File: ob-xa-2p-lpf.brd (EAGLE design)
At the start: 50.8 x 85.5 mm, 53 parts, among them IC1 AS3320, IC3 TL082P

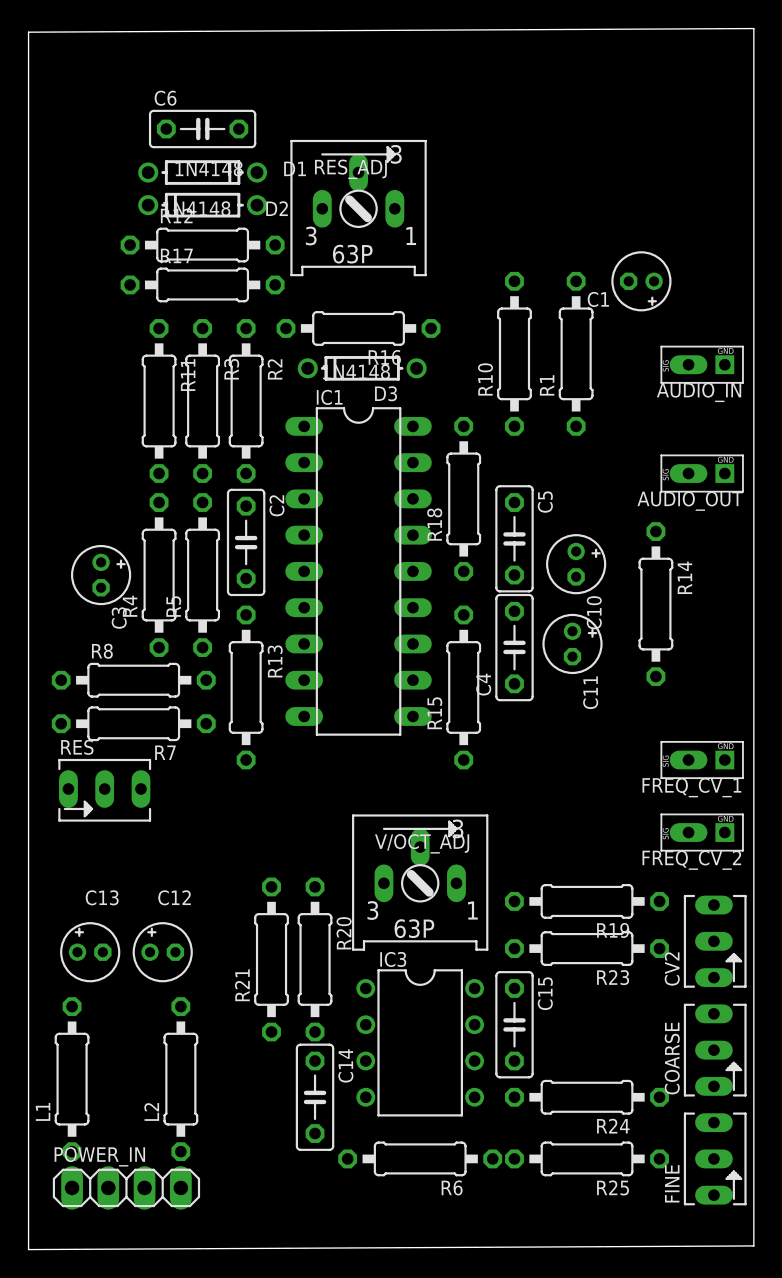
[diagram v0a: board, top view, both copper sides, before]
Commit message: bit more layout cleanup
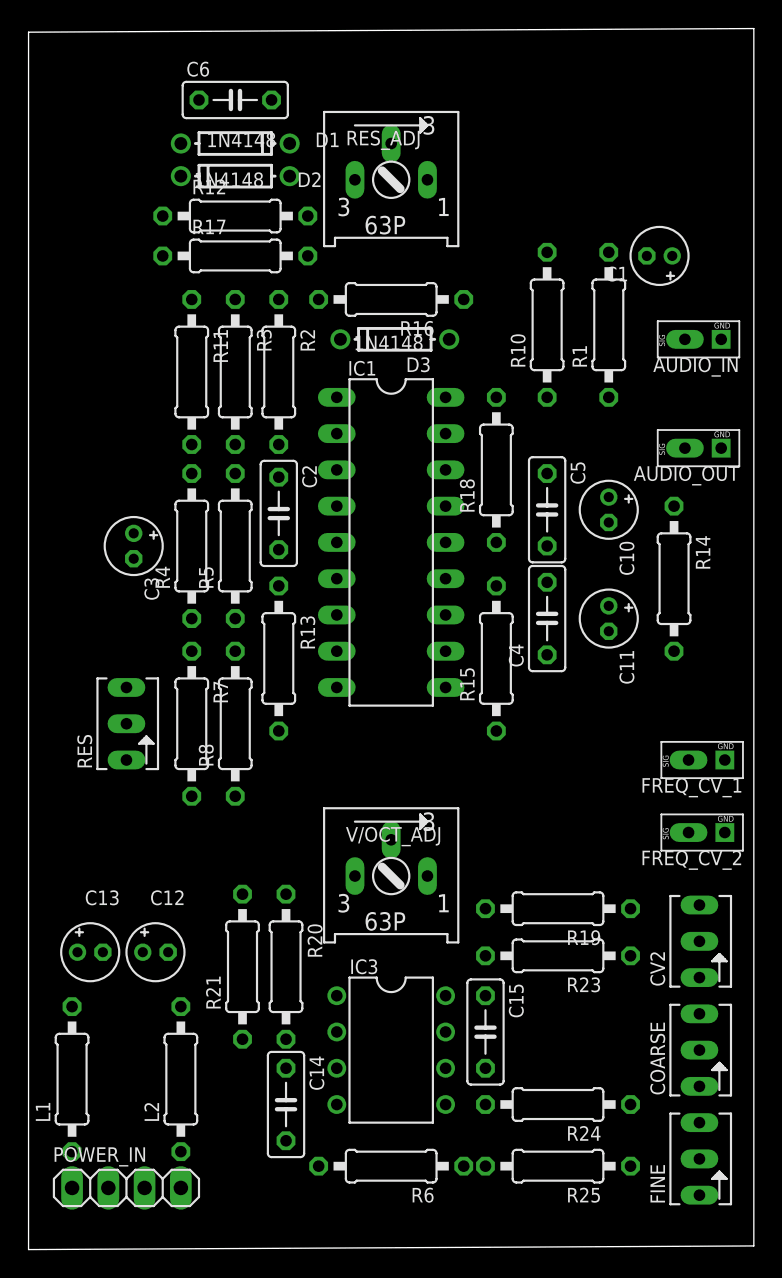
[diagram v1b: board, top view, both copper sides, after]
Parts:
- moved R8 7.74 mm to (14.5, 36.8), turned to 90 degrees
- moved RES 4.82 mm to (6.86, 36.8), turned to 90 degrees
- moved C10 4.44 mm to (40.6, 51.8)
- moved R7 4.06 mm to (11.4, 36.8), turned to 270 degrees
- moved C11 3.10 mm to (40.6, 44.2)
- moved R17 3.06 mm to (14.5, 69.6)
- moved RES_ADJ 3.06 mm to (25.4, 74.9)
- moved C5 3.06 mm to (36.3, 51.8)
- moved C3 3.06 mm to (7.37, 49.3)
- moved R11 3.06 mm to (11.4, 61.5)
- moved R13 3.06 mm to (17.5, 41.4)
- moved R2 3.06 mm to (17.5, 61.5)
- moved R3 3.06 mm to (14.5, 61.5)
- moved R4 3.06 mm to (11.4, 49.3)
- moved R5 3.06 mm to (14.5, 49.3)
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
